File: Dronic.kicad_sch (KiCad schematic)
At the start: 88 parts, among them J1 SWDIO_PH_TERM, J2 Screw_Terminal_01x02, J3 JST_SH_6P_1.00mm, Q1 Q_NMOS, Q10 Q_NMOS, Q11 Q_NMOS, Q12 Q_NMOS, Q13 Q_NMOS, Q14 Q_NMOS, Q15 Q_NMOS, Q16 Q_NMOS, Q17 Q_NMOS, Q18 Q_NMOS, Q19 Q_NMOS, Q2 Q_NMOS, Q20 Q_NMOS, Q21 Q_NMOS, Q22 Q_NMOS, Q23 Q_NMOS, Q24 Q_NMOS, Q25 Q_NMOS, Q26 Q_NMOS, Q3 Q_NMOS, Q4 Q_NMOS, Q5 Q_NMOS, Q6 Q_NMOS, Q7 Q_NMOS, Q8 Q_NMOS, Q9 Q_NMOS, SW1 SW_Push, SW2 SW_Push, U1 RP2040, U2 2137160001, U3 W25Q128JVS, U4 LTC3521EFE-PBF, U5 AP62150WU, U6 ECH8690-TL-H, U7 PCF8575DBR, U8 NTJD5121NT1G, U9 PCF8575DBR, Y1 ABM3B-12.000MHZ-10-1-U-T

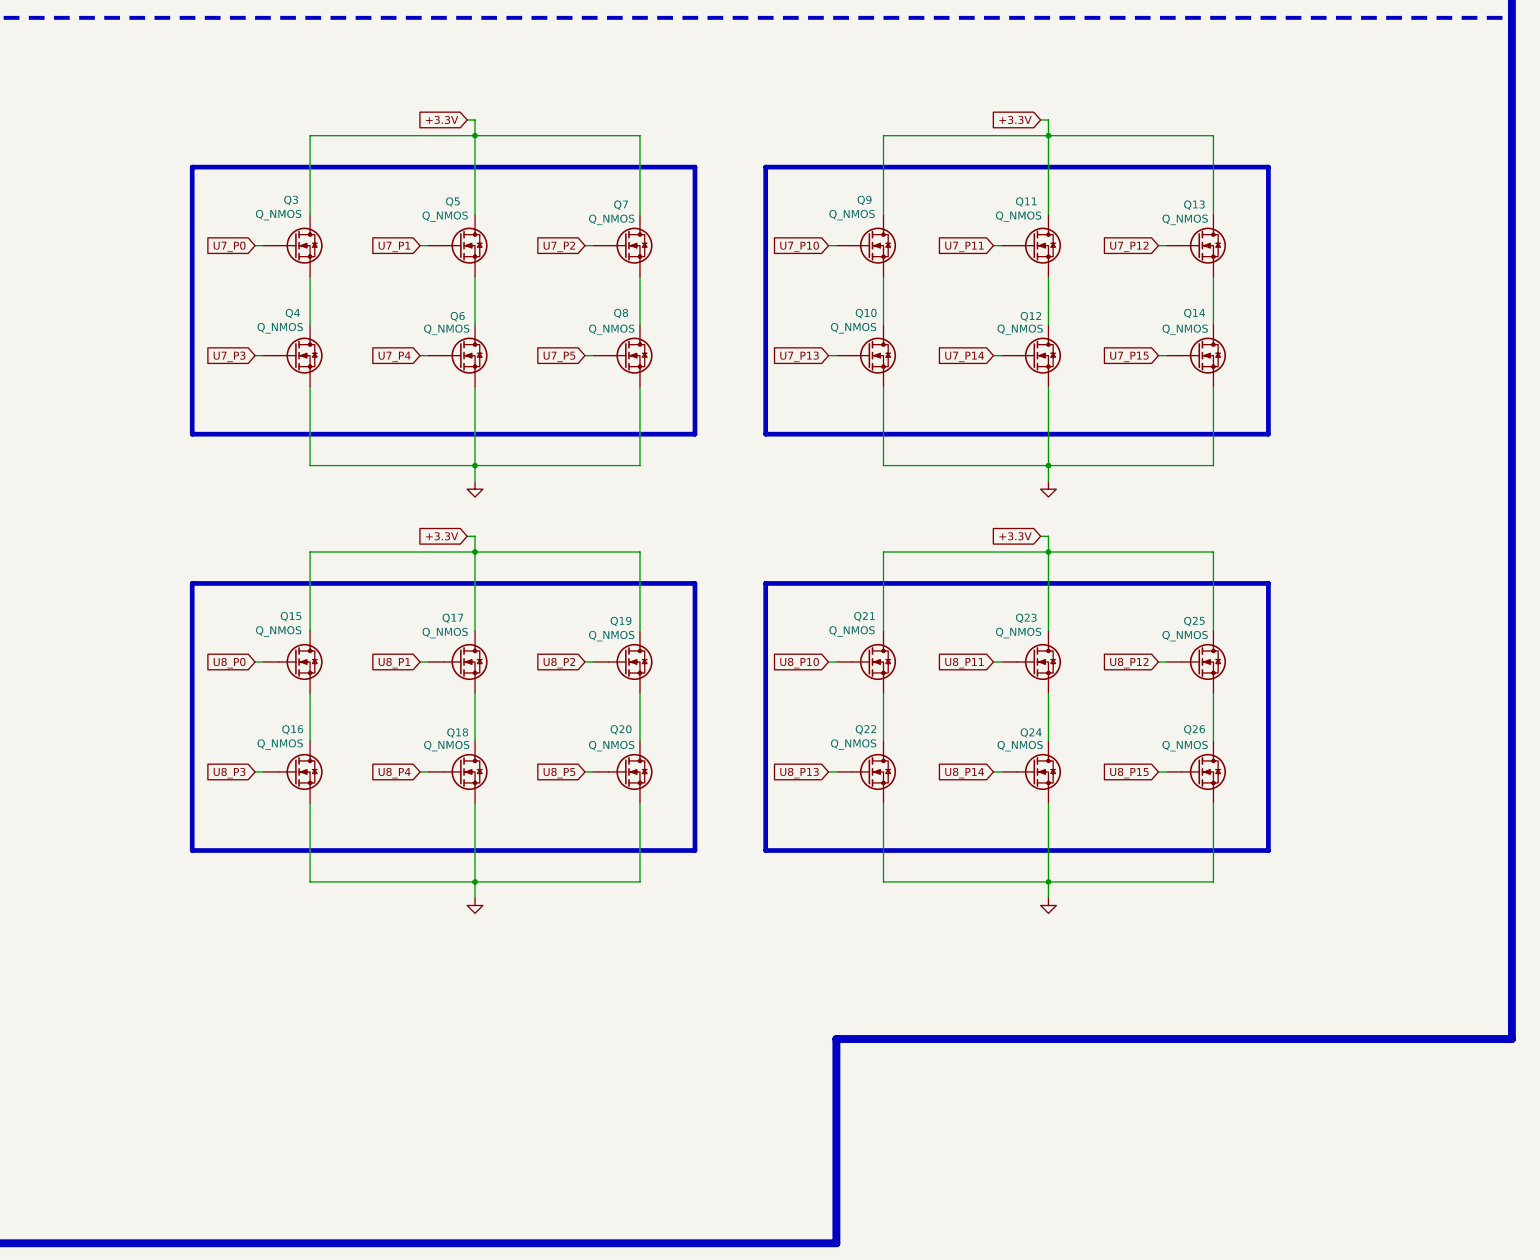
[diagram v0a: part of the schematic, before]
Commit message: Title and Clean Up
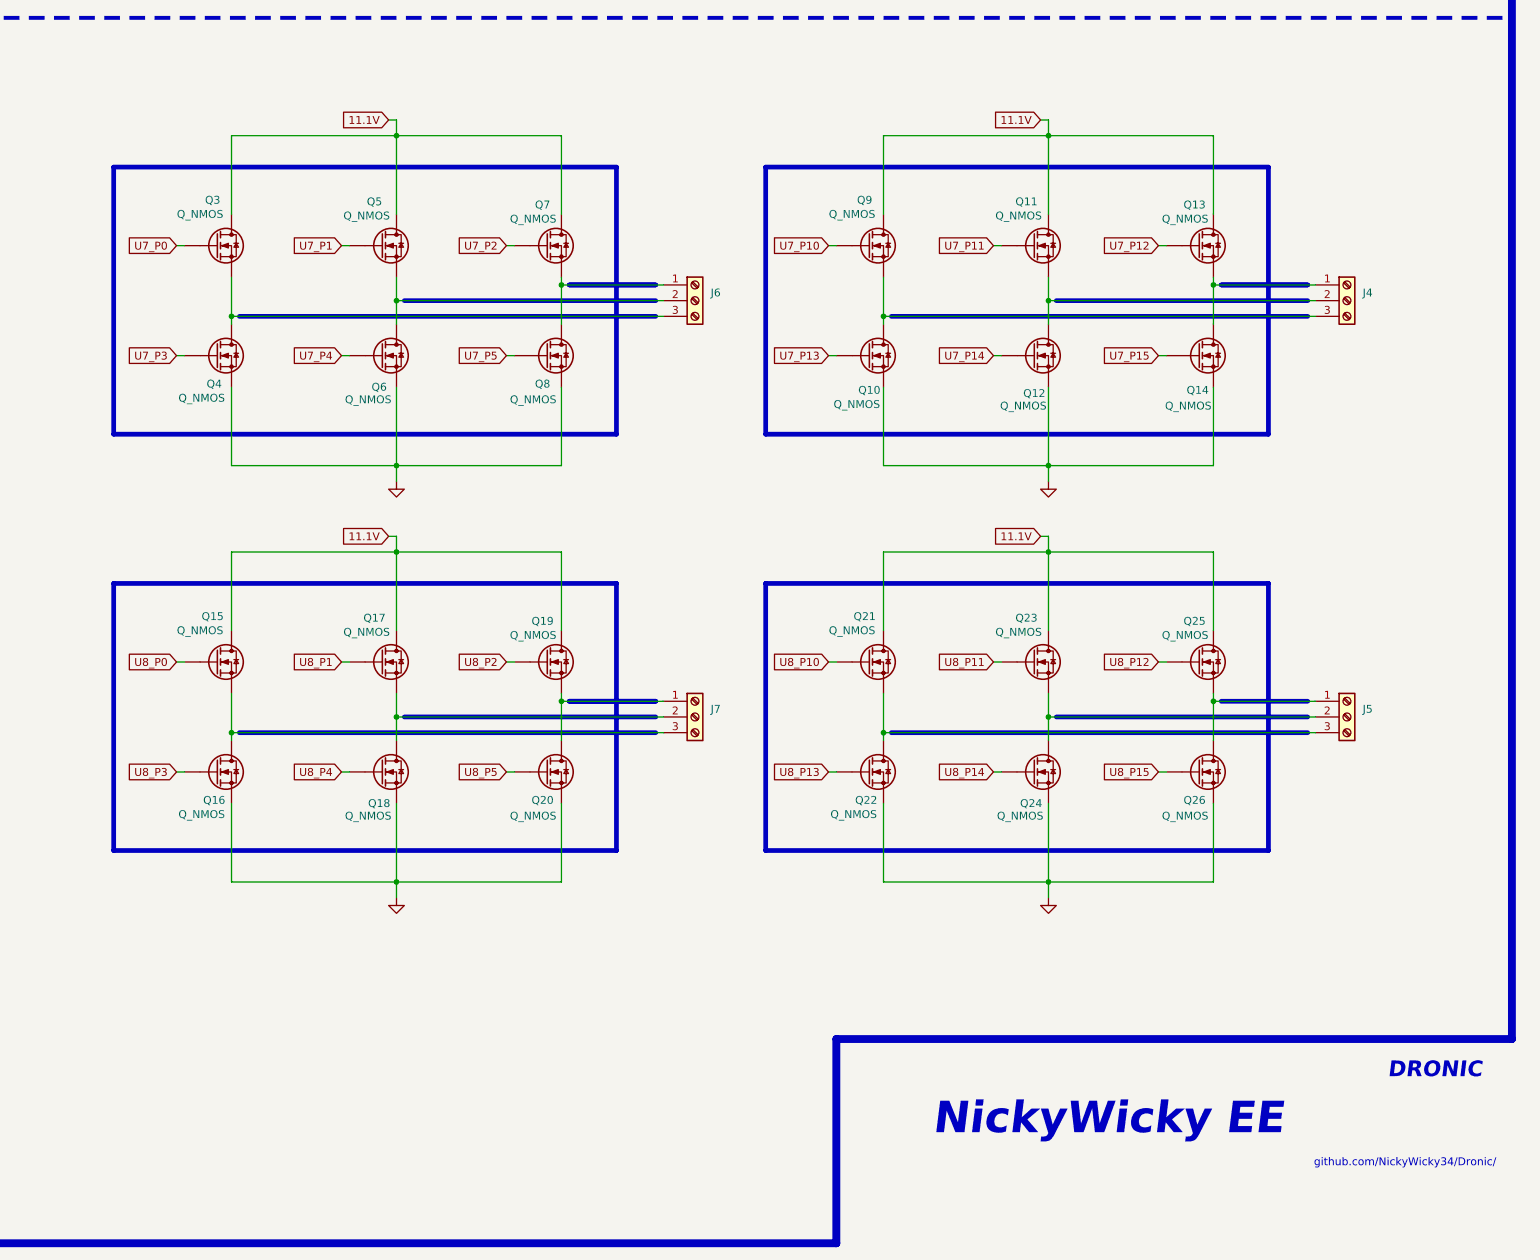
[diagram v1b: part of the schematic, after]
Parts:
- added J4, J5, J6, J7: Screw_Terminal_01x03, symbol Connector:Screw_Terminal_01x03
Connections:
- net +11.1V: now also Q11.D, Q13.D, Q15.D, Q17.D, Q19.D, Q21.D, Q23.D, Q25.D, Q3.D, Q5.D, Q7.D, Q9.D
- net +3.3V: no longer Q11.D, Q13.D, Q15.D, Q17.D, Q19.D, Q21.D, Q23.D, Q25.D, Q3.D, Q5.D, Q7.D, Q9.D
- net at Q21.S, Q22.D: now also J5.3 (Pin_3)
- net at Q5.S, Q6.D: now also J6.2 (Pin_2)
- net at Q15.S, Q16.D: now also J7.3 (Pin_3)
- net at Q7.S, Q8.D: now also J6.1 (Pin_1)
- net at Q19.S, Q20.D: now also J7.1 (Pin_1)
- net at Q11.S, Q12.D: now also J4.2 (Pin_2)
- net at Q13.S, Q14.D: now also J4.1 (Pin_1)
- net at Q10.D, Q9.S: now also J4.3 (Pin_3)
- net at Q17.S, Q18.D: now also J7.2 (Pin_2)
- net at Q23.S, Q24.D: now also J5.2 (Pin_2)
- net at Q25.S, Q26.D: now also J5.1 (Pin_1)
- net at Q3.S, Q4.D: now also J6.3 (Pin_3)
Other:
- note added: "DRONIC"
- note added: "NickyWicky EE"
- note added: "github.com/NickyWicky34/Dronic/"
- moved on the sheet: Q15, Q16, Q17, Q18, Q19, Q20, Q3, Q4, Q5, Q6, Q7, Q8
